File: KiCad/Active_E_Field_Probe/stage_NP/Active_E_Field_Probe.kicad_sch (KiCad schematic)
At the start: 14 parts

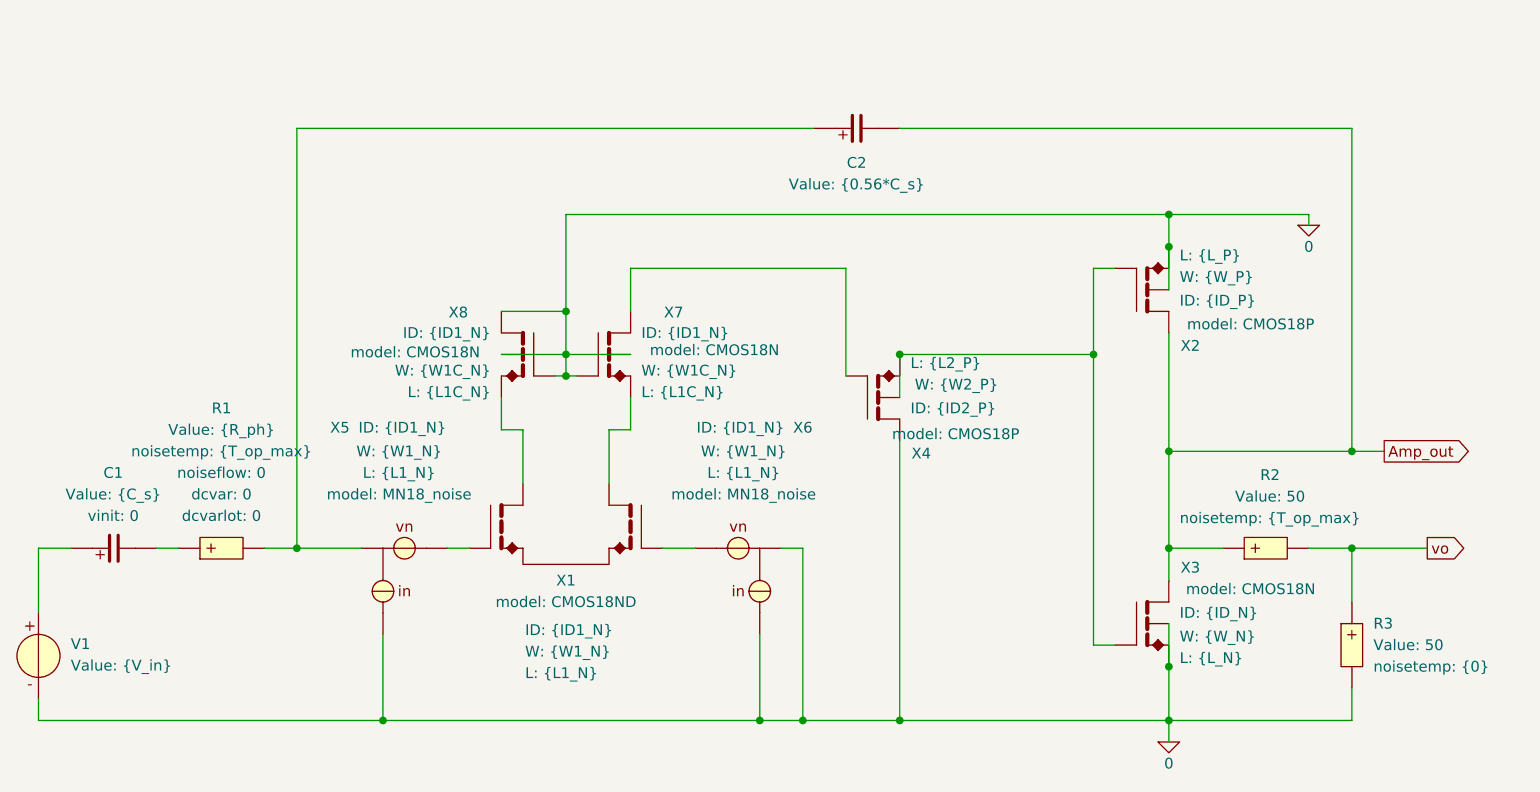
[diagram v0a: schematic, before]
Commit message: diff vf
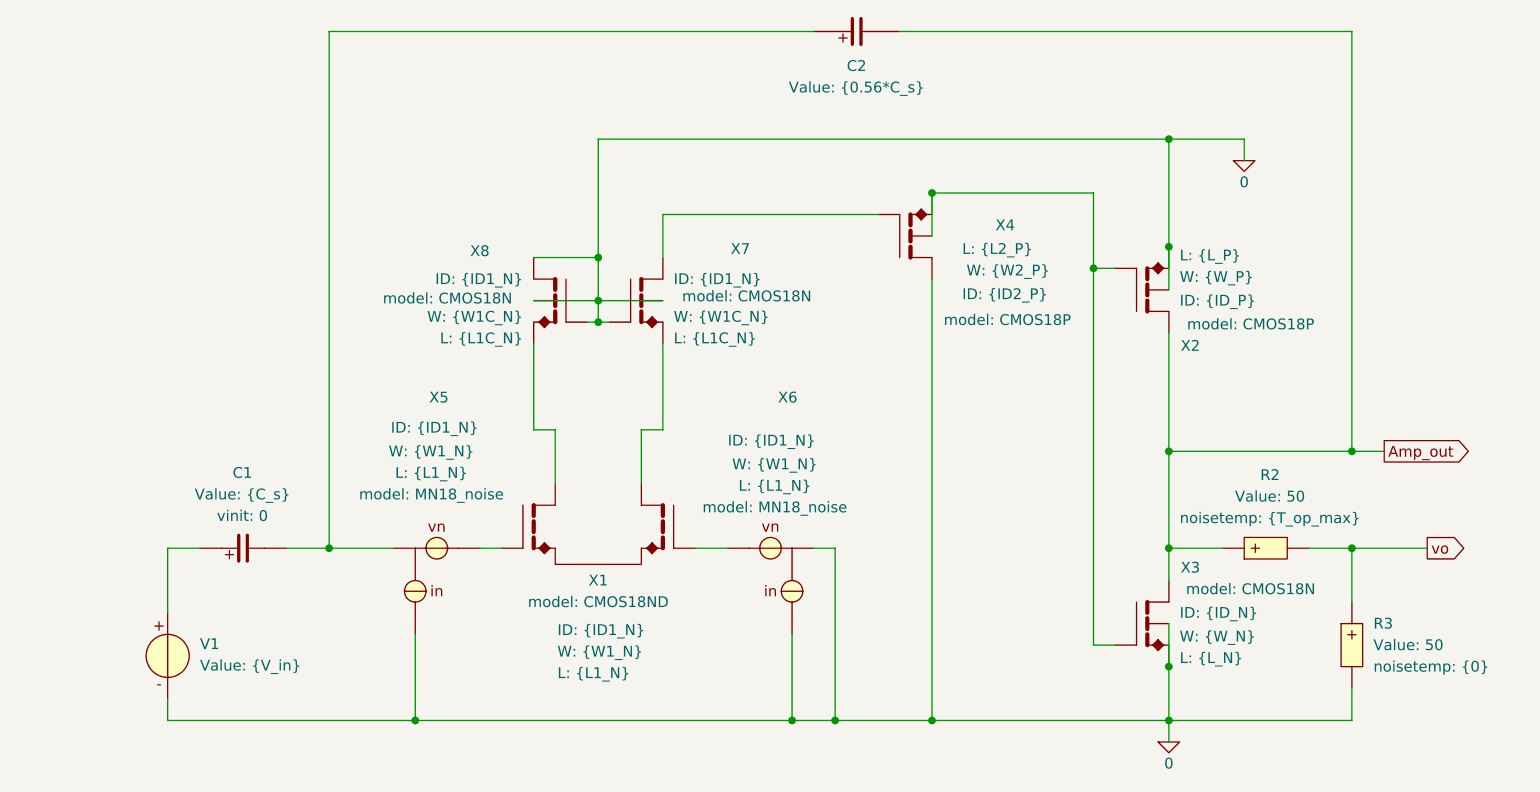
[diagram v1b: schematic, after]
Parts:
- removed R1: {R_ph}, symbol SLiCAP:R
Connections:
- net at C2.1, X5.1 (ext): now also C1.2
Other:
- moved on the sheet: C1, C2, V1, X1, X4, X5, X6, X7, X8
